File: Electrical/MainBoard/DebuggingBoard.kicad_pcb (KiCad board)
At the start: 6 copper layers, 89.9 x 90 mm, 143 parts, among them J1 Barrel_Jack_Switch, Q1 AO3401A, SW1 SW_SPDT, U1 CH224K, U10 FFC2B28-24-G, U11 SM08B-PASS-TBT(LF)(SN), U12 SM05B-PASS-TBT(LF)(SN), U13 SM02B-PASS-TBT(LF)(SN), U14 SM06B-PASS-TBT(LF)(SN), U15 SM05B-PASS-TBT(LF)(SN), U16 SM05B-PASS-TBT(LF)(SN), U17 SM05B-PASS-TBT(LF)(SN), U18 SM05B-PASS-TBT(LF)(SN), U19 SM05B-PASS-TBT(LF)(SN), U2 STM32H723VGTx, U20 SM06B-PASS-TBT(LF)(SN), U22 SM09B-PASS-TBT(LF)(SN), U3 APS6404L-3SQR-ZR, U4 USB3300-EZK, U5 TPS65131RGE, U6 TPS2121RUXR, U7 TPS7A9401DSCR, U8 LM61460AASQRJRRQ1, U9 S5B-ZR-SM4A-TF(LF)(SN), Y1 X322525MOB4SI, Y2 X322524MOB4SI

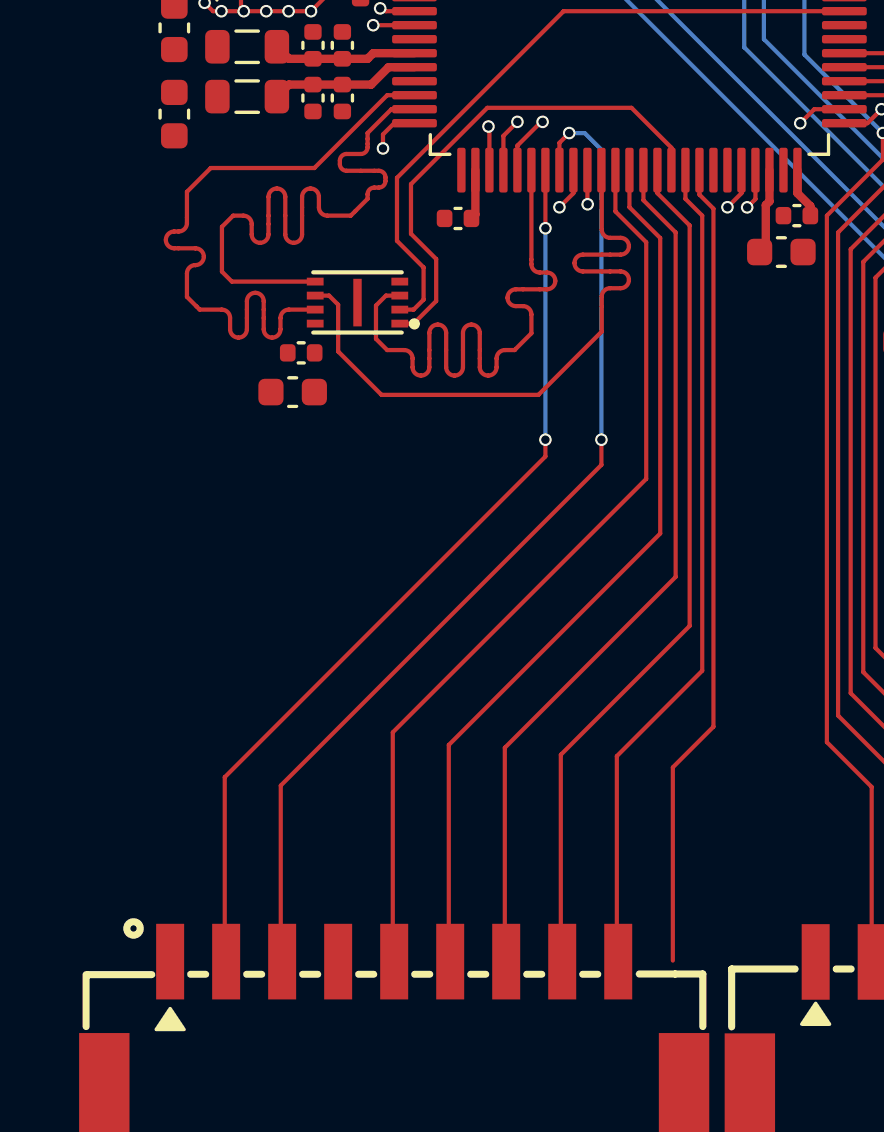
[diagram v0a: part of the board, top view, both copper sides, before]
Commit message: vpsu conn
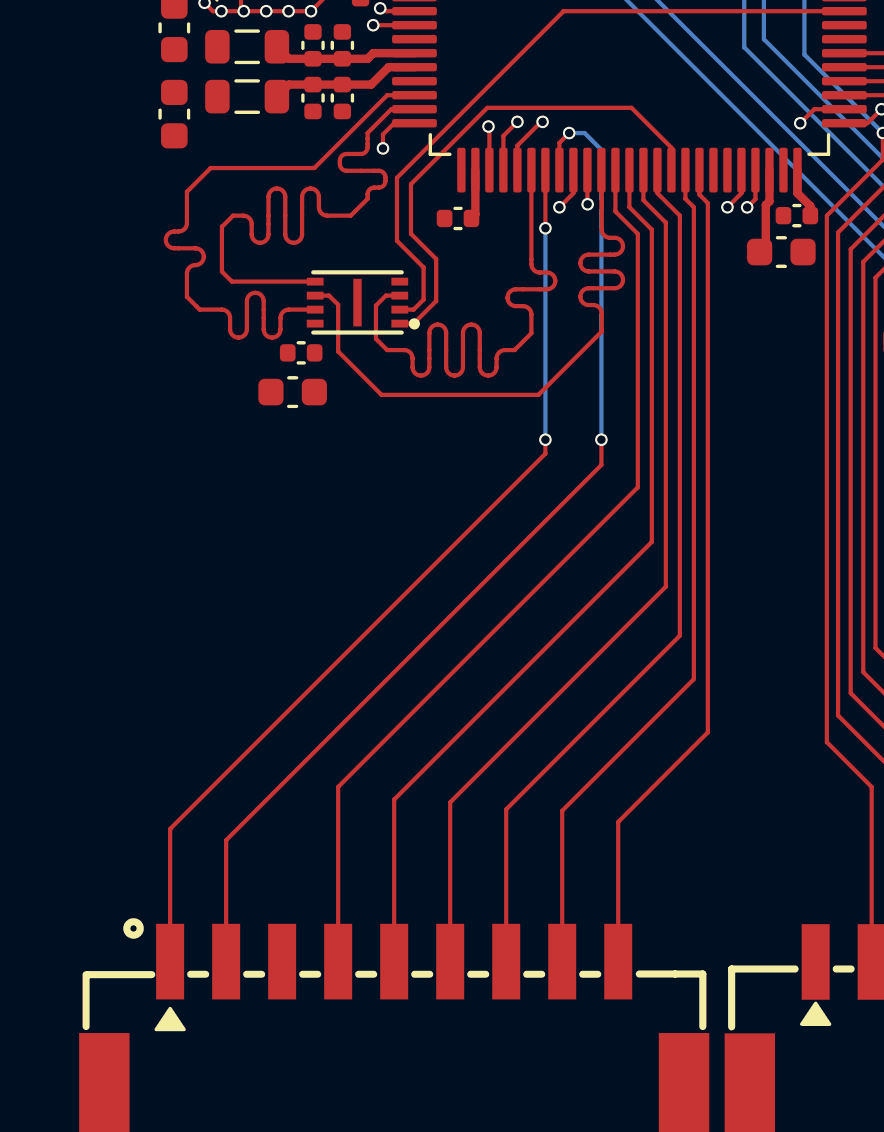
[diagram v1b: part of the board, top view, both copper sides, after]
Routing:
- net /ADC2_INP8: track 36.6 -> 37.4 mm
- net /ADC1_INP4: track 33.0 -> 33.8 mm
- net /BUZZER_CTRL: track 29.0 -> 29.7 mm
- net /MULT_CONN_IND: track 29.7 -> 30.3 mm
- net /R_SRC_100K: track 31.8 -> 32.4 mm
- net /R_SRC_1K: track 32.4 -> 33.0 mm
- net /V_RANGE_LOW: track 31.2 -> 31.8 mm
- net /V_RANGE_HIGH: track 30.6 -> 31.2 mm
